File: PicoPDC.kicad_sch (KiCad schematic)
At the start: 56 parts, among them J1 DE15_Pins_HighDensity, J10 Conn_02x10_Odd_Even, J11 DB25_Socket, J2 To PICO, J3 Conn_02x04_Odd_Even, J4 Conn_01x01_Pin, J5 Micro_SD_Card, J6 To ProgDC, J8 W5500 Lite, J9 DB25_Pins, U1 RASPBERRY_PI_PICO, U2 SN74LVC8T245, U3 74LS30, U4 74AHCT125, U5 74LS30, U6 RASPBERRY_PI_PICO, U7 74LS373, U8 74LVC1G32

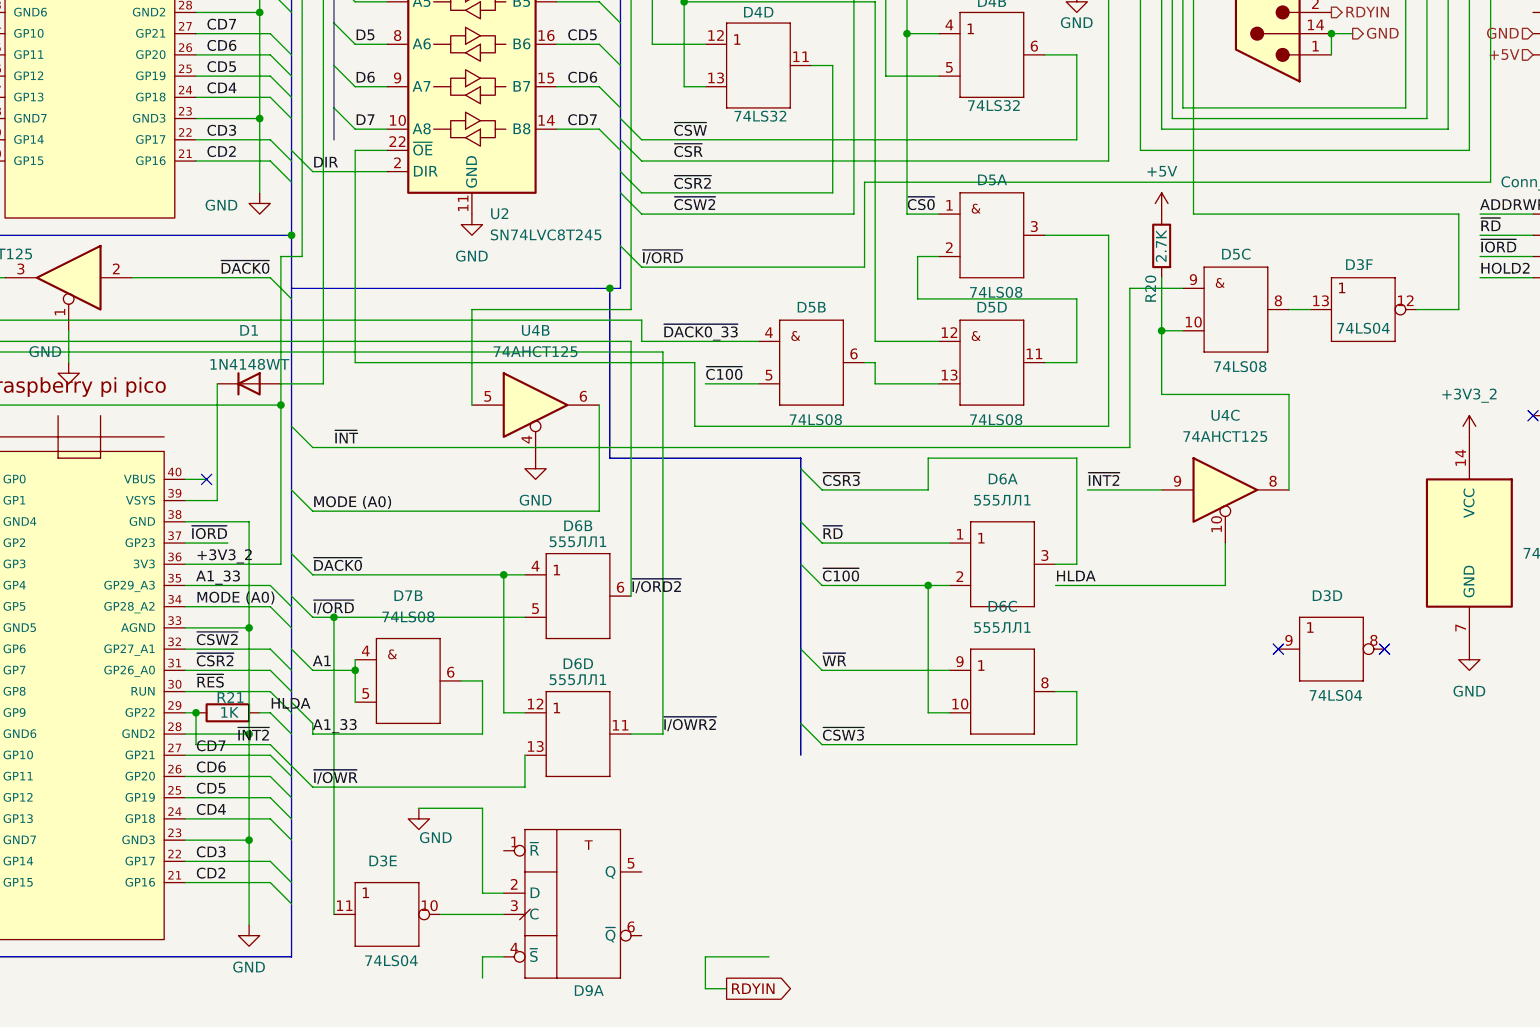
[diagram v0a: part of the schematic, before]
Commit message: Update
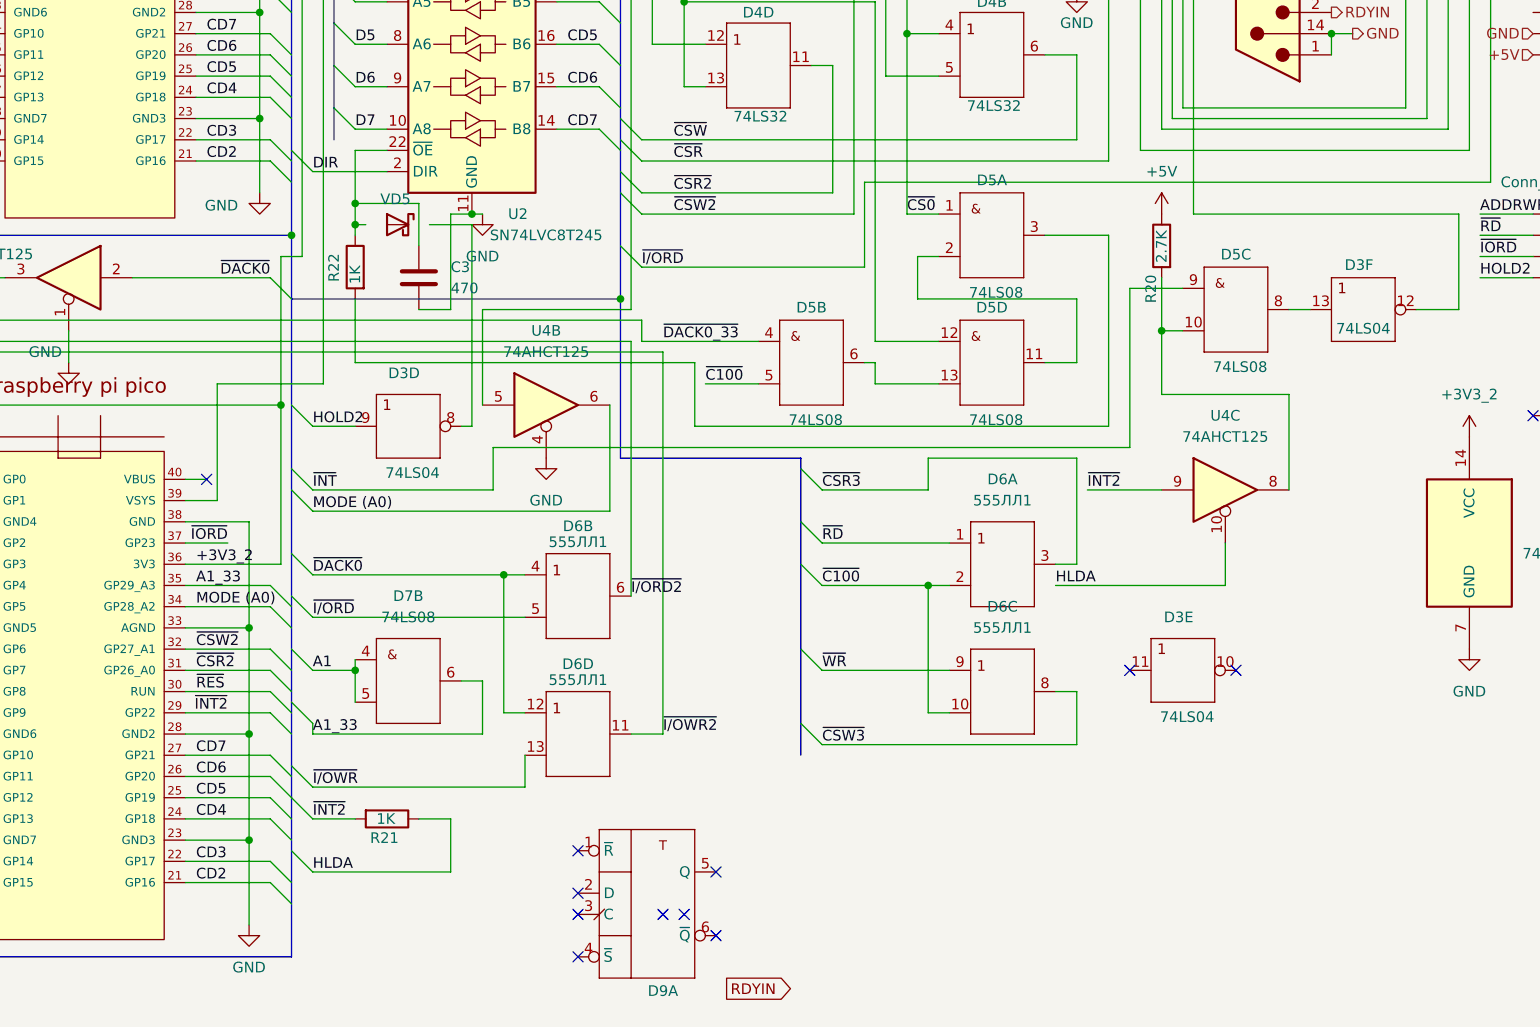
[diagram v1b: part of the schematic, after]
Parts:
- removed D1: 1N4148WT, Diode_SMD:D_SOD-523, symbol Diode:1N4148WT
- added C3: 470, Capacitor_THT:C_Rect_L7.0mm_W2.0mm_P5.00mm, symbol Device:C
- added R22: 1K, Resistor_THT:R_Axial_DIN0207_L6.3mm_D2.5mm_P5.08mm_Vertical, symbol Device:R
- added VD5: 1N4148, Diode_THT:D_DO-34_SOD68_P2.54mm_Vertical_AnodeUp, symbol Diode:BAT43
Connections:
- net +5V: now also U6.39 (VSYS)
- net GND: now also C3.2; no longer D9.2 (D)
- net HLDA: now also R21.1; no longer R21.2
- net HOLD2: now also D3.9 (A)
- net ~{I/ORD}: no longer D3.11 (A)
- net ~{INT2}: now also R21.2; no longer R21.1
- net at D3.10 (Y): no longer D9.3 (C)
- net at U2.22 (~{OE}): now also C3.1, R22.1; no longer D5.3 (Y)
- new net: D5.3 (Y), R22.2
- no-connect marks 23 -> 31
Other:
- moved on the sheet: U4B
